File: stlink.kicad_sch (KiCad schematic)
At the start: 36 parts, among them CON4 USB_C_Wurth_632723300011, Q1 BC847B, U5 STM32F103C(8-B)Tx, U6 MCP1700T-3302E_MB, X1 8.000MHZ

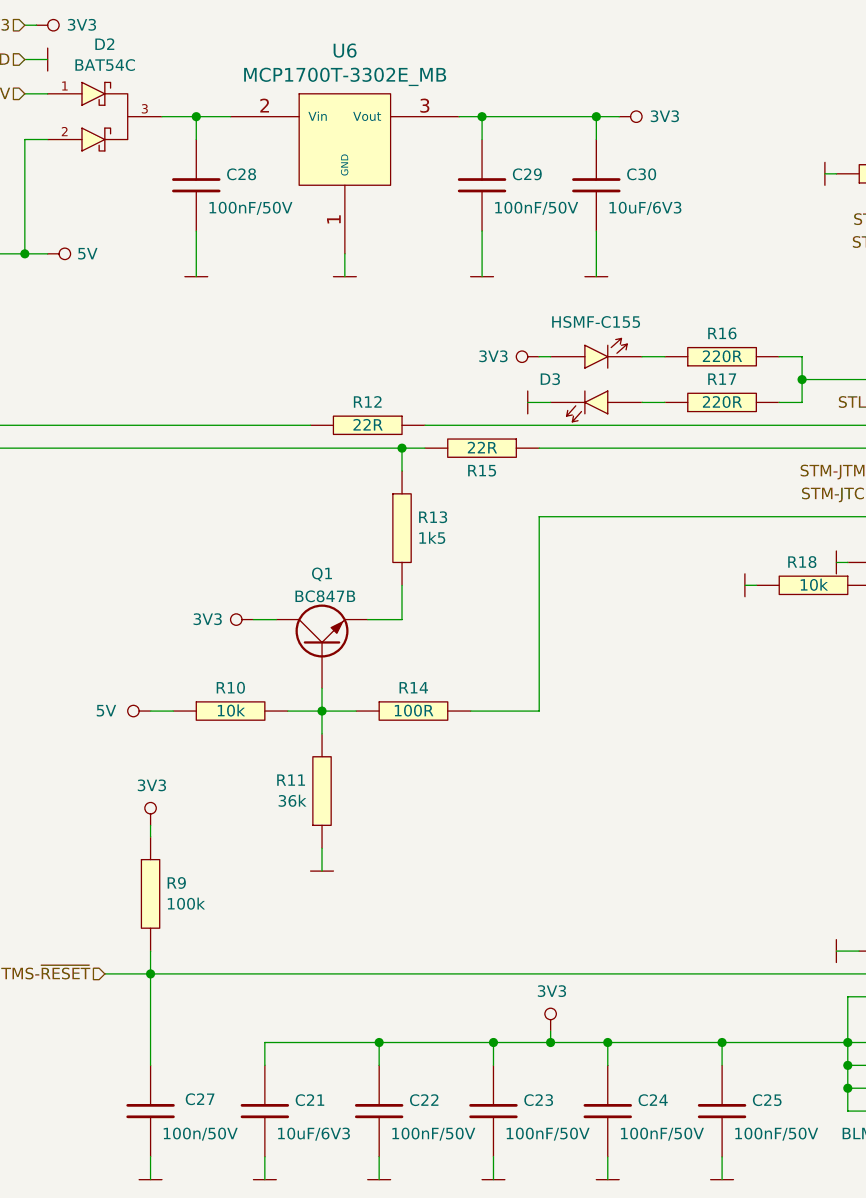
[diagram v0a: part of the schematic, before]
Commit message: Gerbers created, BOM, CPL
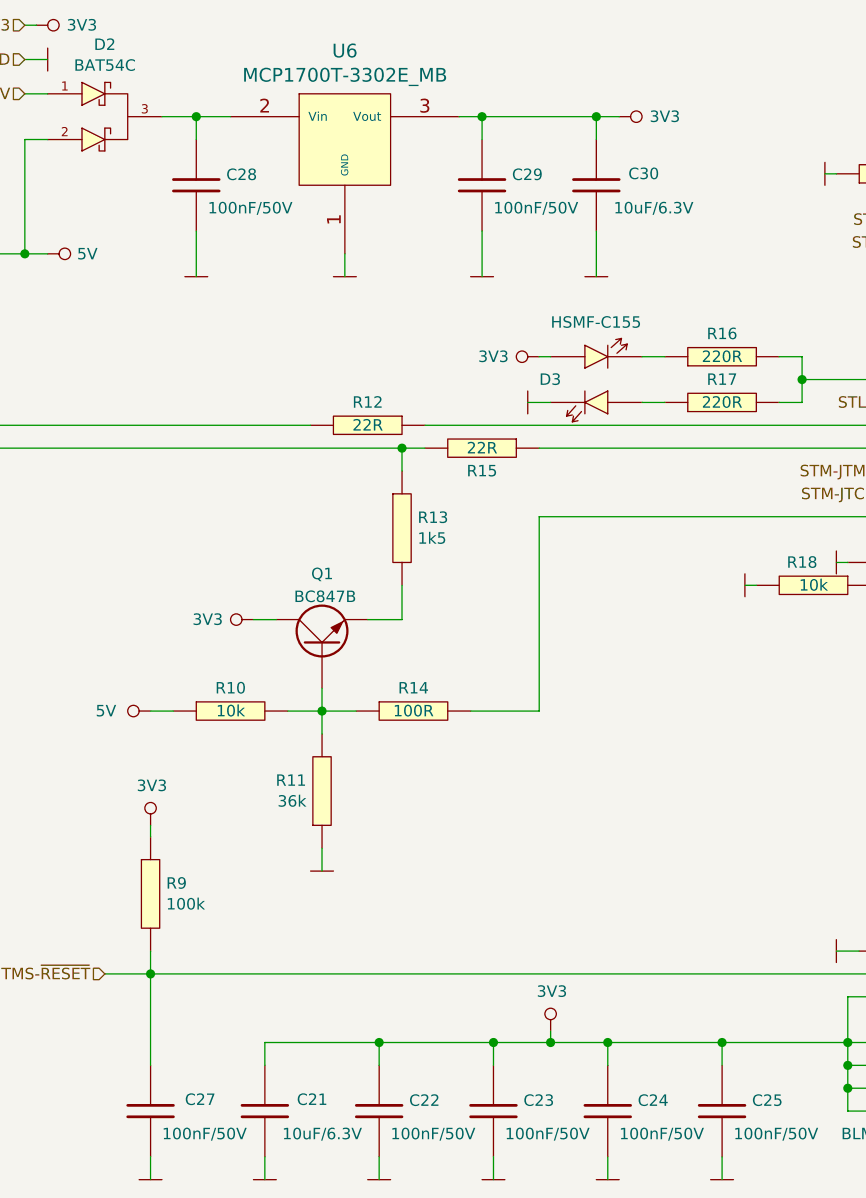
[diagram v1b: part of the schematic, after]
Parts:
- removed C21, C30: 10uF/6V3, Capacitors_Smd_0805:10uF_0805, symbol Capacitors_Smd0805:10uF_6V3
- added C21, C30: 10uF/6.3V, Capacitors_Smd_0603:10uF_10V_0603, symbol Capacitors_Smd0603:10uF
- C27: value 100n/50V -> 100nF/50V
- R21, R9: Price@1pcs (none) -> 0,07415
- U6: Developer WP -> MW; LCSC Part #(optional) (none) -> C632000; Package (none) -> SOT89
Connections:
- net 3V3: now also C21.1, C30.1
- net GND: now also C21.2, C30.2
